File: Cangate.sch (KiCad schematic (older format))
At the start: 1 part

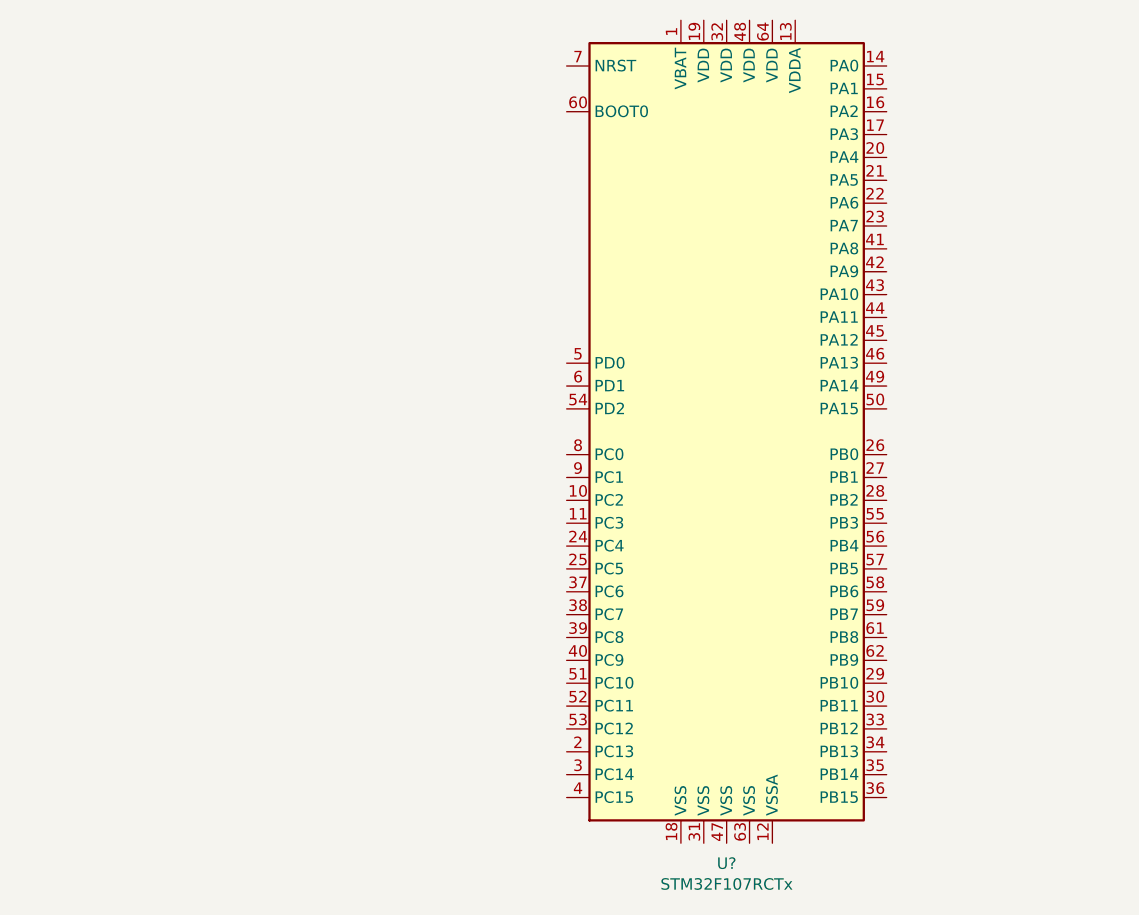
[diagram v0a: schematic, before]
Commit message: Cangate Index Scheme
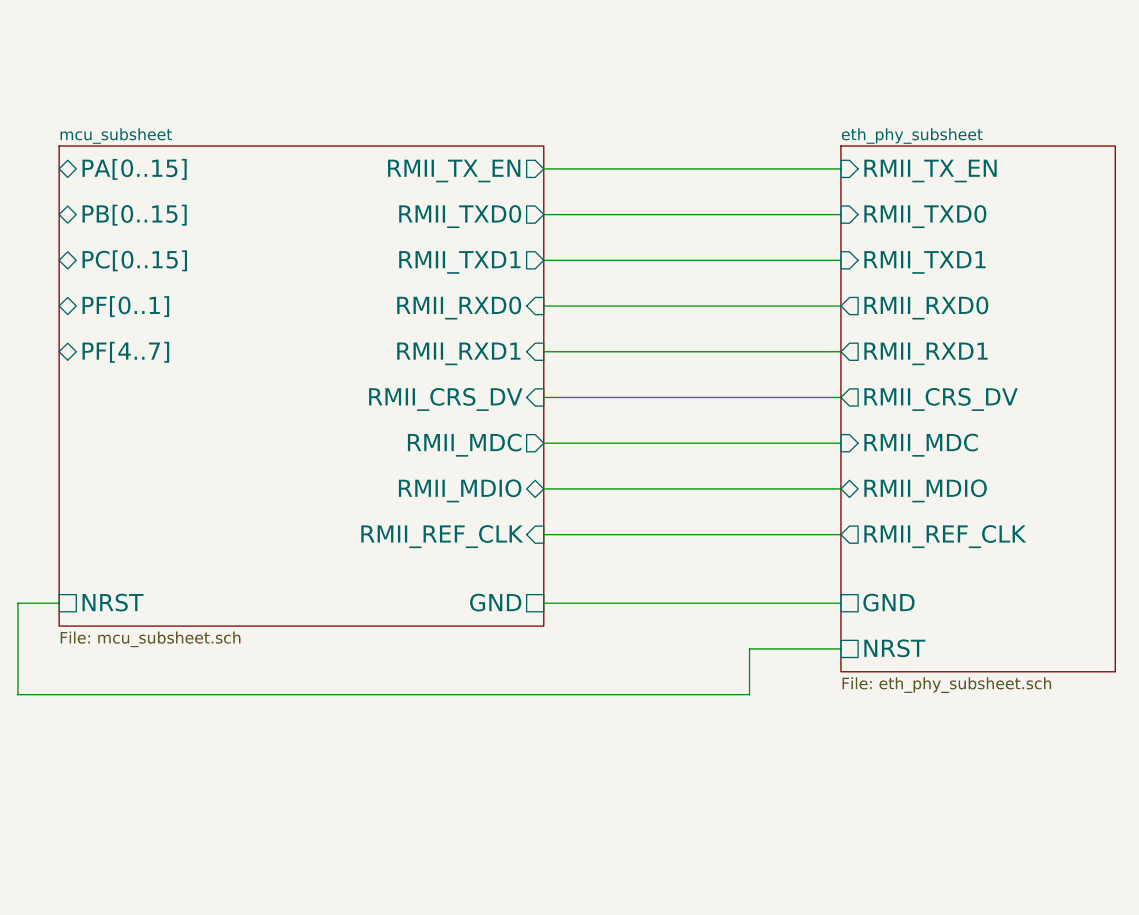
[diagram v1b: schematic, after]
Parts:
- removed U?: STM32F107RCTx, Package_QFP:LQFP-64_10x10mm_P0.5mm, symbol MCU_ST_STM32F1:STM32F107RCTx
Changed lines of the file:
@@
 $Descr A4 11693 8268
 encoding utf-8
-Sheet 1 1
+Sheet 1 3
 Title "Cangate"
 Date "2021-10-24"
@@
 Comment4 "Author: Tsekhavoi Ivan"
 $EndDescr
-$Comp
-L MCU_ST_STM32F1:STM32F107RCTx U?
-U 1 1 6175CB2B
-P 5600 3850
-F 0 "U?" H 5600 1961 50  0000 C CNN
-F 1 "STM32F107RCTx" H 5600 1870 50  0000 C CNN
-F 2 "Package_QFP:LQFP-64_10x10mm_P0.5mm" H 5000 2150 50  0001 R CNN
-F 3 "http://www.st.com/st-web-ui/static/active/en/resource/technical/document/datasheet/CD00220364.pdf" H 5600 3850 50  0001 C CNN
-	1    5600 3850
-	1    0    0    -1
-$EndComp
+$Sheet
+S 6100 2600 1200 2300
+U 6176B826
+F0 "eth_phy_subsheet" 50
+F1 "eth_phy_subsheet.sch" 50
+F2 "RMII_TX_EN" I L 6100 2700 75
+F3 "RMII_TXD0" I L 6100 2900 75
+F4 "RMII_TXD1" I L 6100 3100 75
+F5 "RMII_RXD0" O L 6100 3300 75
+F6 "RMII_RXD1" O L 6100 3500 75
+F7 "RMII_CRS_DV" O L 6100 3700 75
+F8 "RMII_MDC" I L 6100 3900 75
+F9 "RMII_MDIO" B L 6100 4100 75
+F10 "RMII_REF_CLK" O L 6100 4300 75
+F11 "GND" U L 6100 4600 75
+F12 "NRST" U L 6100 4800 75
+$EndSheet
+$Sheet
+S 2680 2600 2120 2100
+U 6176B761
+F0 "mcu_subsheet" 50
+F1 "mcu_subsheet.sch" 50
+F2 "RMII_TX_EN" O R 4800 2700 75
+F3 "RMII_TXD0" O R 4800 2900 75
+F4 "RMII_TXD1" O R 4800 3100 75
+F5 "RMII_RXD0" I R 4800 3300 75
+F6 "RMII_RXD1" I R 4800 3500 75
+F7 "RMII_CRS_DV" I R 4800 3700 75
+F8 "RMII_MDC" O R 4800 3900 75
+F9 "RMII_MDIO" B R 4800 4100 75
+F10 "RMII_REF_CLK" I R 4800 4300 75
+F11 "GND" U R 4800 4600 75
+F12 "NRST" U L 2680 4600 75
+F13 "PA[0..15]" B L 2680 2700 75
+F14 "PB[0..15]" B L 2680 2900 75
+F15 "PC[0..15]" B L 2680 3100 75
+F16 "PF[0..1]" B L 2680 3300 75
+F17 "PF[4..7]" B L 2680 3500 75
+$EndSheet
+Wire Wire Line
+	4800 2700 6100 2700
+Wire Wire Line
+	4800 2900 6100 2900
+Wire Wire Line
+	4800 3100 6100 3100
+Wire Wire Line
+	4800 3300 6100 3300
+Wire Wire Line
+	4800 3700 6100 3700
+Wire Wire Line
+	6100 3500 4800 3500
+Wire Wire Line
+	4800 3900 6100 3900
+Wire Wire Line
+	6100 4100 4800 4100
+Wire Wire Line
+	6100 4300 4800 4300
+Wire Wire Line
+	4800 4600 6100 4600
+Wire Wire Line
+	6100 4800 5700 4800
+Wire Wire Line
+	5700 4800 5700 5000
+Wire Wire Line
+	5700 5000 2500 5000
+Wire Wire Line
+	2500 5000 2500 4600
+Wire Wire Line
+	2500 4600 2680 4600
 $EndSCHEMATC
